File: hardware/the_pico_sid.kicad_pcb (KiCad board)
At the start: 4 copper layers, 18.8 x 38.6 mm, 40 parts, among them J1 Conn_01x06, Q1 2N7002, Q2 2N7002, U1 SID_6581, U2 RP2040, U3 AMS1117-3.3, U4 W25Q16JVS, U5 LM324, U6 4050, U7 4050, U8 74HC245, Y1 12MHz

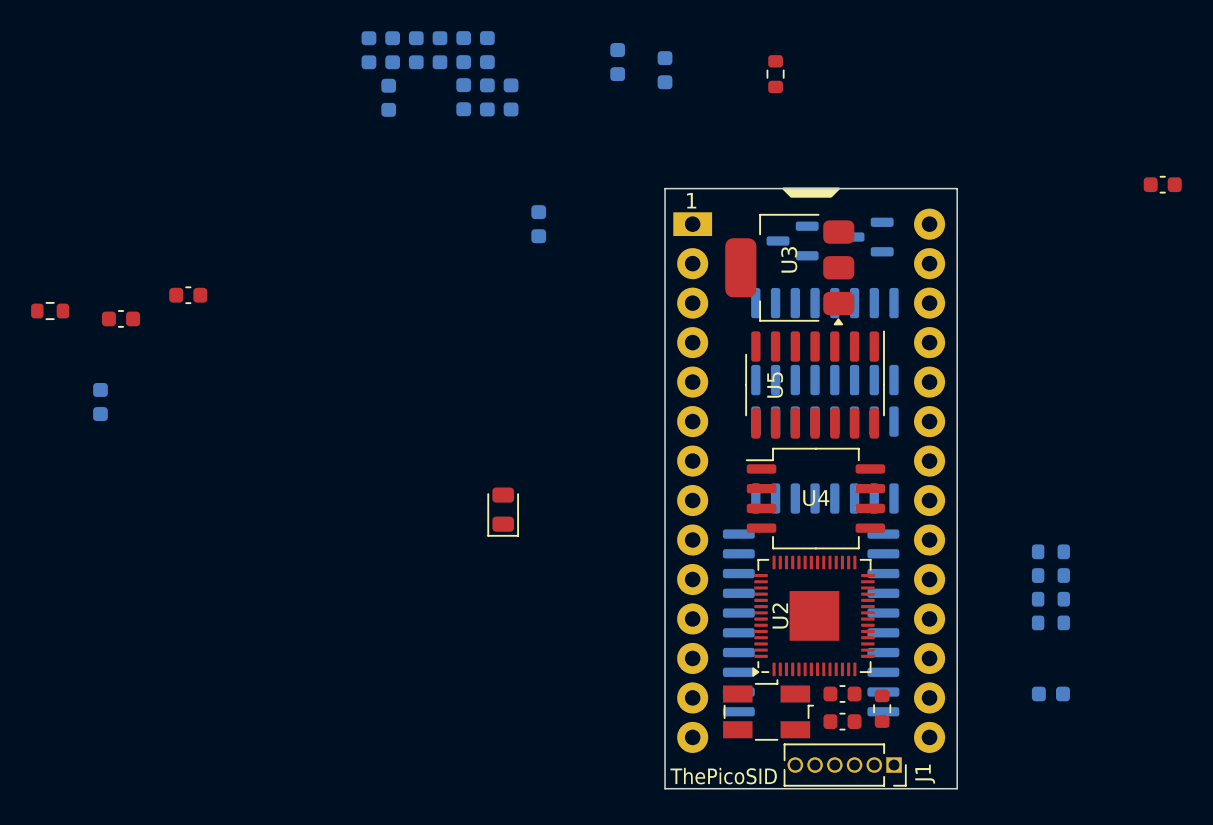
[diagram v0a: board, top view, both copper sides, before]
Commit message: new pcb and gerber files for JLCPCB production
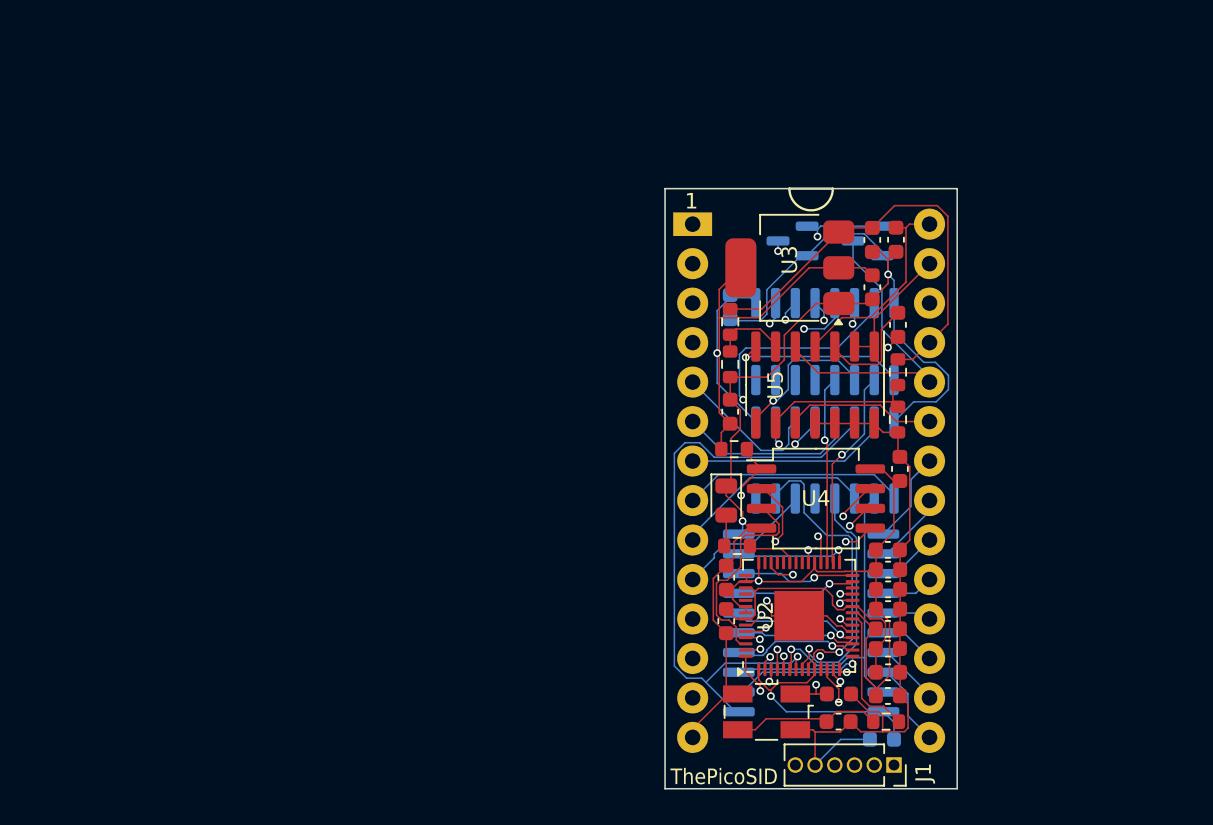
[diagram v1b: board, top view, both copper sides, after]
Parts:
- C1, C10, C11, C12, C16, C19, C2, C3, C4, C5, C6, C7, C8, C9, R4, R5, R6, R7: moved to F.Cu
- C18: moved to B.Cu
- moved C6 52.4 mm to (152.5, 110.9), turned to 0 degrees
- moved C17 50.0 mm to (153.2, 87.0), turned to 90 degrees
- moved C5 48.0 mm to (152.5, 106.6), turned to 0 degrees
- moved C13 47.1 mm to (153.3, 96.3), turned to 90 degrees
- moved R1 46.7 mm to (142.8, 101.2)
- moved C1 46.3 mm to (152.5, 101.5), turned to 0 degrees
- moved C4 46.1 mm to (152.5, 105.3), turned to 0 degrees
- moved C10 44.2 mm to (152.5, 109.3), turned to 0 degrees
- moved C3 44.1 mm to (152.5, 104.0), turned to 0 degrees
- moved C9 43.8 mm to (152.5, 107.8), turned to 0 degrees
- moved C2 42.2 mm to (152.5, 102.7), turned to 0 degrees
- moved C19 40.5 mm to (142.4, 92.6)
- moved C18 40.0 mm to (152.1, 113.7)
- moved C8 37.7 mm to (142.1, 103.3), turned to 90 degrees
- moved C20 32.3 mm to (142.4, 85.9), turned to 90 degrees
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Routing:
- net GND: track 0.00 -> 139.6 mm, vias 0 -> 3
- net +3.3V: track 0.00 -> 112.8 mm, vias 0 -> 3
- net RW: track 0.00 -> 39.8 mm, vias 0 -> 1
- net A4_C64: track 0.00 -> 33.9 mm, vias 0 -> 1
- net A3: track 0.00 -> 31.6 mm, vias 0 -> 2
- net +5V: track 0.00 -> 28.1 mm
- net A3_C64: track 0.00 -> 27.4 mm, vias 0 -> 1
- net A2: track 0.00 -> 27.2 mm, vias 0 -> 2
- net ADC_2KHZ: track 0.00 -> 26.5 mm, vias 0 -> 2
- net A4: track 0.00 -> 26.3 mm, vias 0 -> 2
- net POTY: track 0.00 -> 26.0 mm, vias 0 -> 1
- net A2_C64: track 0.00 -> 23.1 mm, vias 0 -> 1
- net POTX: track 0.00 -> 20.8 mm
- net AUDIO_PWM: track 0.00 -> 20.0 mm, vias 0 -> 2
- net CS: track 0.00 -> 20.0 mm, vias 0 -> 1
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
